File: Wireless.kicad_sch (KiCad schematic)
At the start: 37 parts, among them J11 Conn_01x02_Pin, J16 Conn_01x04_Pin, J17 Conn_01x04_Pin, SW6 SW_Push, SW7 SW_Push, U14 ESP32-C3FH4, Y2 40MHz

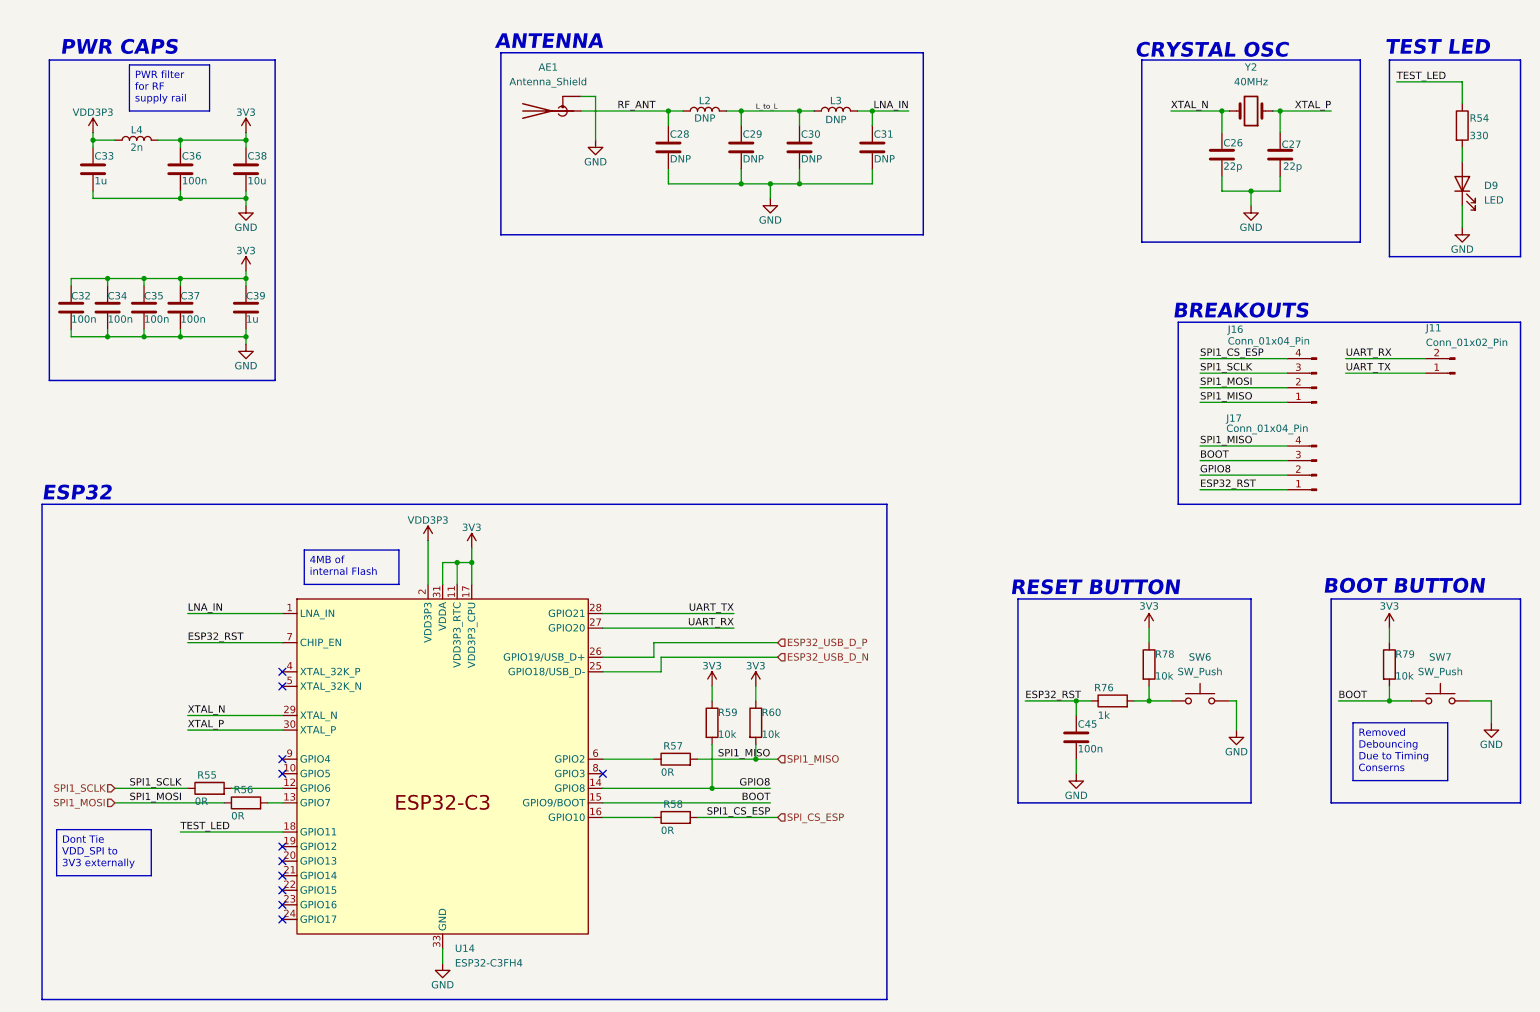
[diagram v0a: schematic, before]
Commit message: small changes
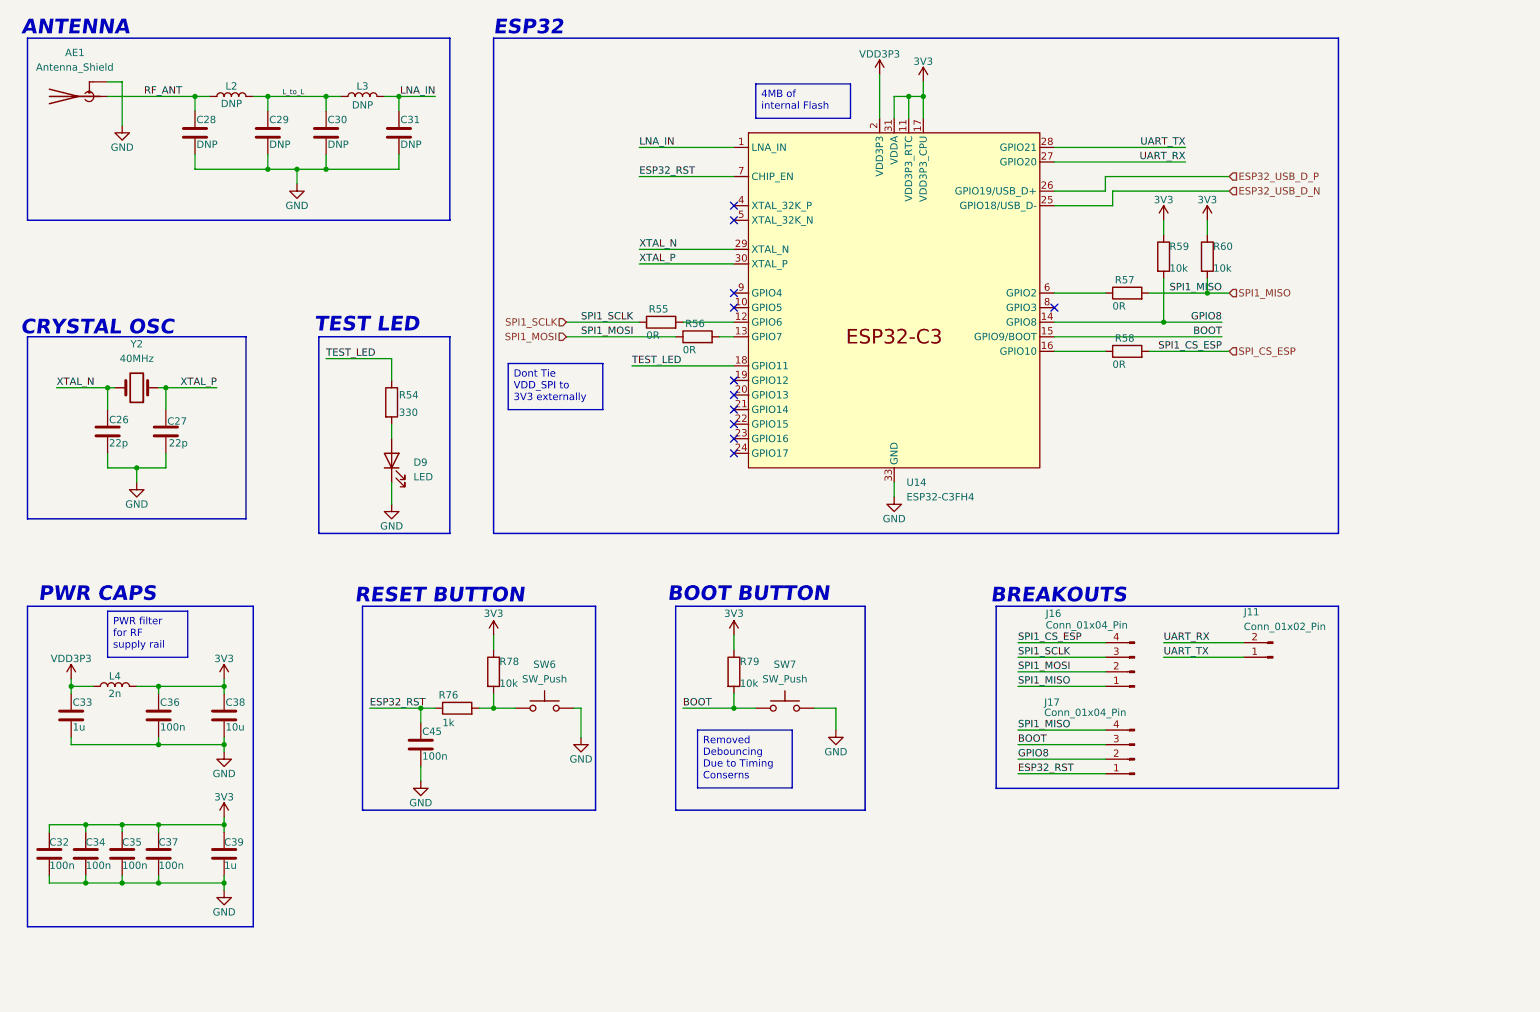
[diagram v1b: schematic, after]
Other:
- moved on the sheet: AE1, C26, C27, C28, C29, C30, C31, C32, C33, C34, C35, C36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
